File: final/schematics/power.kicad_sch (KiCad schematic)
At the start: 4 parts, among them J1 B2B-PH-K-S, U11 MP2161GJ-Z, U12 LT3045EMSE_PBF, U13 LTC3122EMSE_PBF

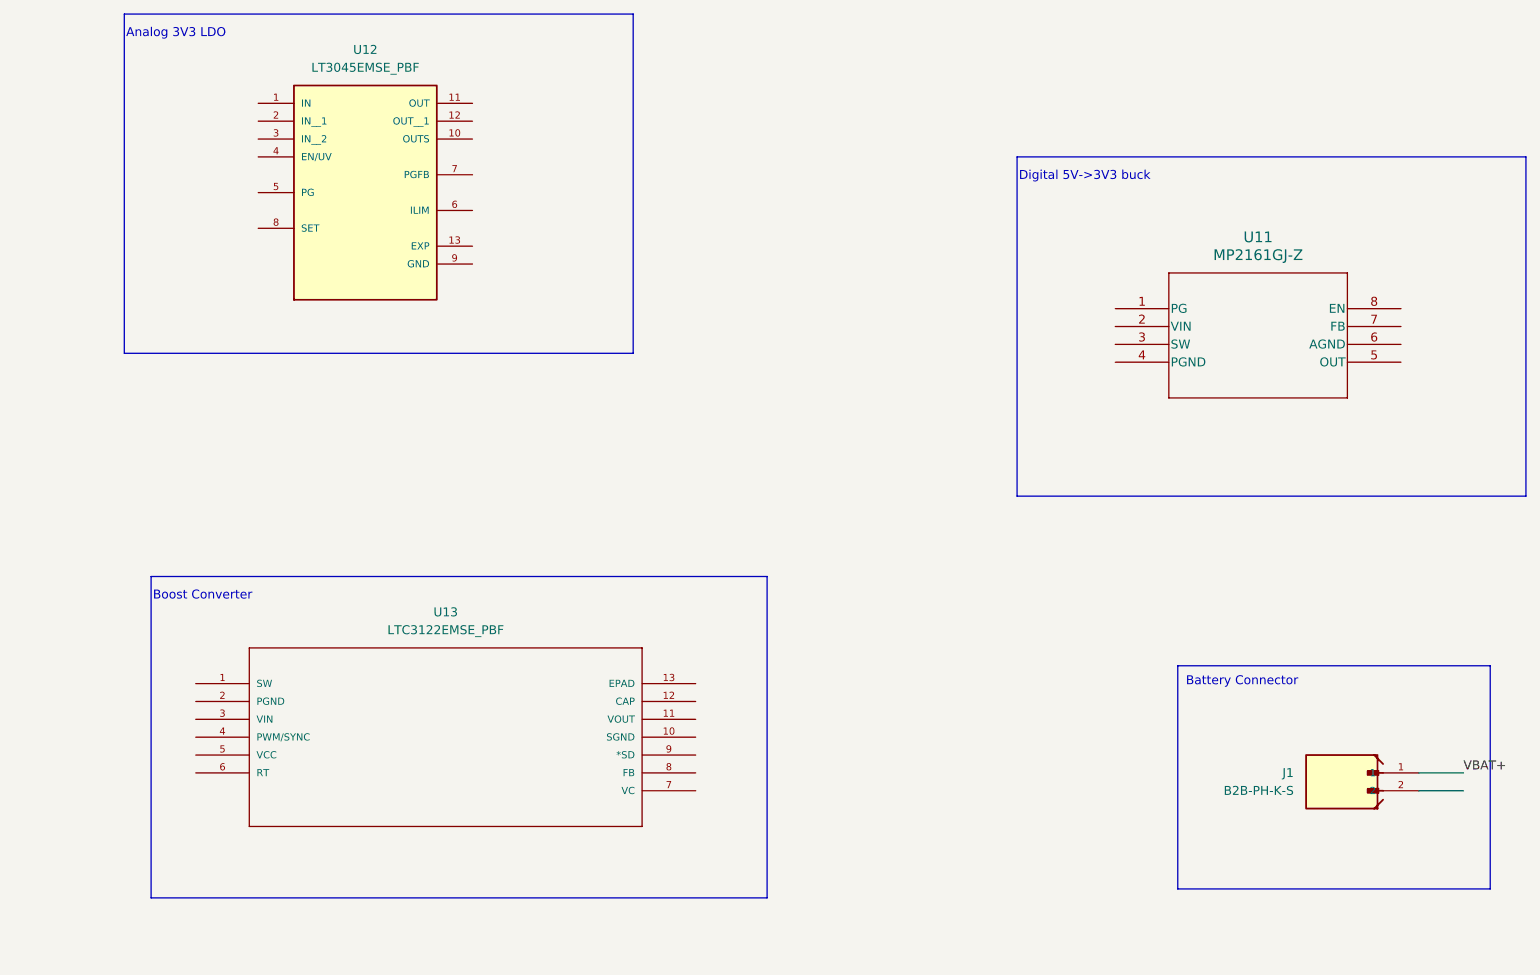
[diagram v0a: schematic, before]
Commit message: finishing
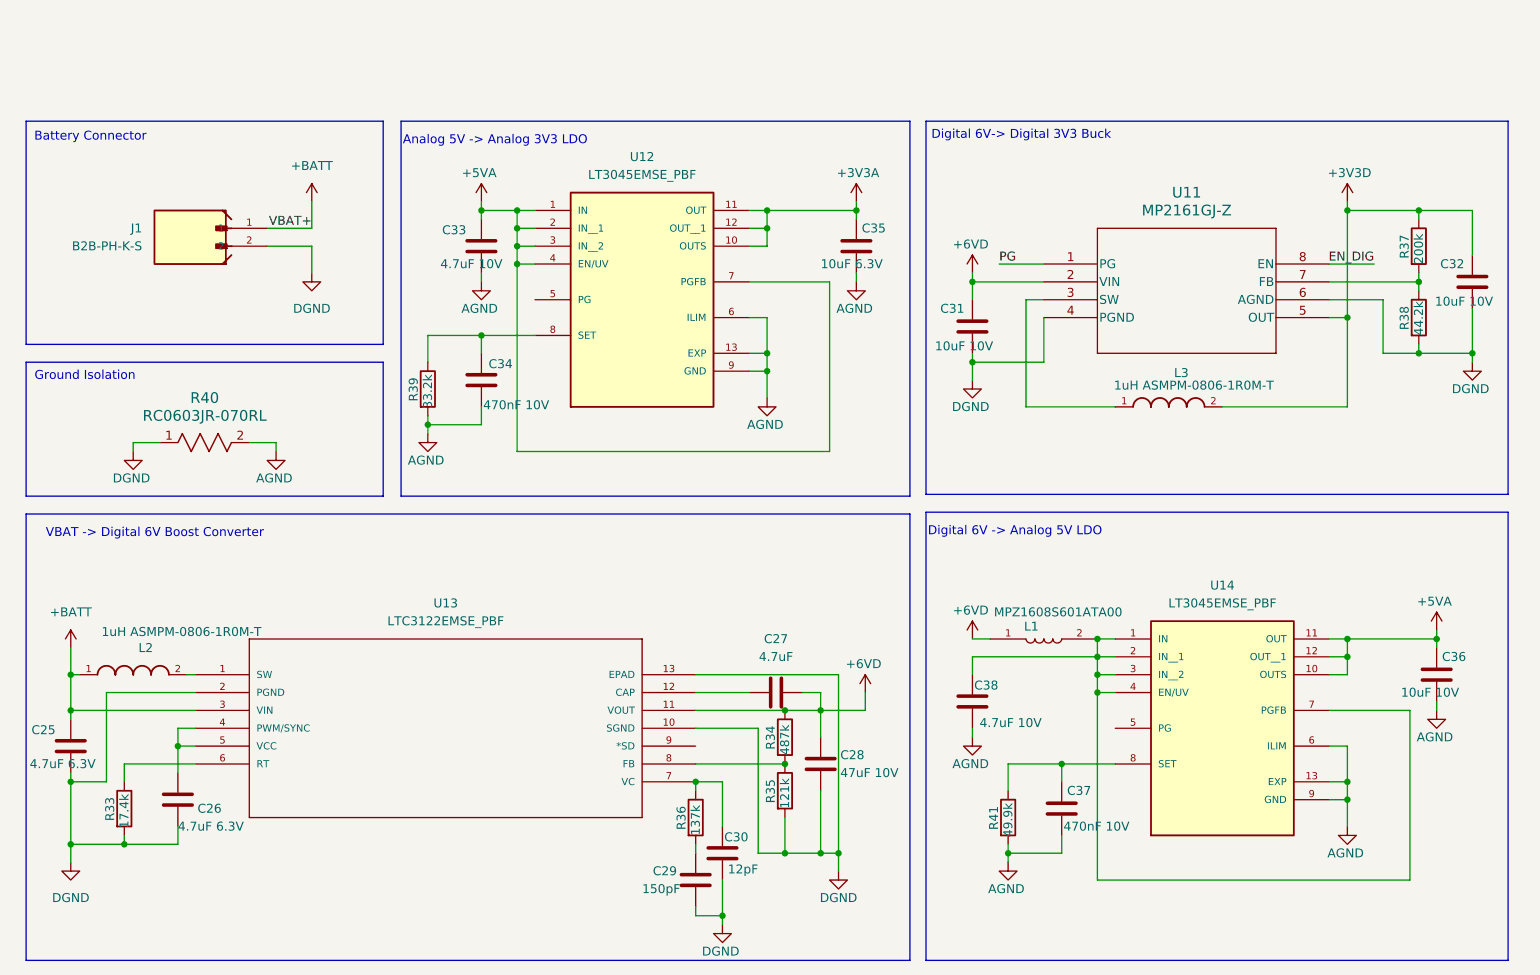
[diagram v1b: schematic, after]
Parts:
- added C25: 4.7uF 6.3V, Capacitor_SMD:C_1206_3216Metric, symbol Device:C
- added C26: 4.7uF 6.3V, Capacitor_SMD:C_0603_1608Metric, symbol Device:C
- added C27: 4.7uF, Capacitor_SMD:C_0603_1608Metric, symbol Device:C
- added C28: 47uF 10V, Capacitor_SMD:C_1206_3216Metric, symbol Device:C
- added C29: 150pF, Capacitor_SMD:C_0603_1608Metric, symbol Device:C
- added C30: 12pF, Capacitor_SMD:C_0603_1608Metric, symbol Device:C
- added C31, C32, C36: 10uF 10V, Capacitor_SMD:C_1206_3216Metric, symbol Device:C
- added C33, C38: 4.7uF 10V, Capacitor_SMD:C_1206_3216Metric, symbol Device:C
- added C34, C37: 470nF 10V, Capacitor_SMD:C_1206_3216Metric, symbol Device:C
- added C35: 10uF 6.3V, Capacitor_SMD:C_1206_3216Metric, symbol Device:C
- added L1: MPZ1608S601ATA00, MPZ1608S601ATA00:INDC1608X95N, symbol MPZ1608S601ATA00:MPZ1608S601ATA00
- added L2, L3: 1uH ASMPM-0806-1R0M-T, ASMPM_0806_1R0M_T:INDC2016X100N, symbol ASMPM-0806-1R0M-T:ASMPM-0806-1R0M-T
- added R33: 17.4k, Resistor_SMD:R_0603_1608Metric, symbol Device:R
- added R34: 487k, Resistor_SMD:R_0603_1608Metric, symbol Device:R
- added R35: 121k, Resistor_SMD:R_0603_1608Metric, symbol Device:R
- added R36: 137k, Resistor_SMD:R_0603_1608Metric, symbol Device:R
- added R37: 200k, Resistor_SMD:R_0603_1608Metric, symbol Device:R
- added R38: 44.2k, Resistor_SMD:R_0603_1608Metric, symbol Device:R
- added R39: 33.2k, Resistor_SMD:R_0603_1608Metric, symbol Device:R
- added R40: RC0603JR-070RL, RC0603N_YAG, symbol RC0603JR_070RL:RC0603JR-070RL
- added R41: 49.9k, Resistor_SMD:R_0603_1608Metric, symbol Device:R
- added U14: LT3045EMSE_PBF, LT3045EMSE_PBF:SOP65P490X110-13N, symbol LT3045EMSE_PBF:LT3045EMSE_PBF
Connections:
- net VBAT+ is gone; now on net +BATT: J1.1
- net +5VA: now reaches U12.1 (IN)
- net +5VA: now also U12.2 (IN__1), U12.3 (IN__2), U12.4 (EN/UV), U12.7 (PGFB), C33.1, C36.1, U14.10 (OUTS), U14.11 (OUT), U14.12 (OUT__1)
- net +3V3A: now reaches U12.10 (OUTS)
- net +3V3A: now also U12.11 (OUT), U12.12 (OUT__1), C35.1
- net AGND: now reaches U12.13 (EXP)
- net AGND: now also U12.6 (ILIM), U12.9 (GND), C33.2, C34.2, C35.2, C36.2, C37.2, C38.2, R39.2, R40.2, R41.2, U14.13 (EXP), U14.6 (ILIM), U14.9 (GND)
- net at U12.8 (SET): now also C34.1, R39.1
- net DGND: now reaches J1.2
- net DGND: now also U11.4 (PGND), U11.6 (AGND), U13.10 (SGND), U13.13 (EPAD), U13.2 (PGND), C25.2, C26.2, C28.1, C29.1, C30.1, C31.1, C32.1, R33.2, R35.2, R38.2, R40.1
- net at U13.1 (SW): now also L2.2
- net +6VD: now reaches U13.11 (VOUT)
- net +6VD: now also U11.2 (VIN), C27.2, C28.2, C31.2, L1.1, R34.1
- net at U13.12 (CAP): now also C27.1
- net +BATT: now reaches U13.3 (VIN)
- net +BATT: now also C25.1, L2.1
- net at U13.4 (PWM/SYNC): now also U13.5 (VCC), C26.1
- net at U13.6 (RT): now also R33.1
- net at U13.7 (VC): now also C30.2, R36.1
- net at U13.8 (FB): now also R34.2, R35.1
- net PG: now reaches U11.1 (PG)
- net at U11.3 (SW): now also L3.1
- net +3V3D: now reaches U11.5 (OUT)
- net +3V3D: now also C32.2, L3.2, R37.1
- net at U11.7 (FB): now also R37.2, R38.1
- net EN_DIG: now reaches U11.8 (EN)
- new net: C37.1, R41.1, U14.8 (SET)
- new net: C38.1, L1.2, U14.1 (IN), U14.2 (IN__1), U14.3 (IN__2), U14.4 (EN/UV), U14.7 (PGFB)
- new net: C29.2, R36.2
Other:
- note added: "Analog 5V -> Analog 3V3 LDO"
- note added: "Digital 6V -> Analog 5V LDO"
- note added: "Digital 6V-> Digital 3V3 Buck"
- note added: "Ground Isolation"
- note added: "VBAT -> Digital 6V Boost Converter"
- note removed: "Analog 3V3 LDO"
- note removed: "Boost Converter"
- note removed: "Digital 5V->3V3 buck"
- moved on the sheet: J1, U11, U12, U13
